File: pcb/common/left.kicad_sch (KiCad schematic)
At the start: 87 parts

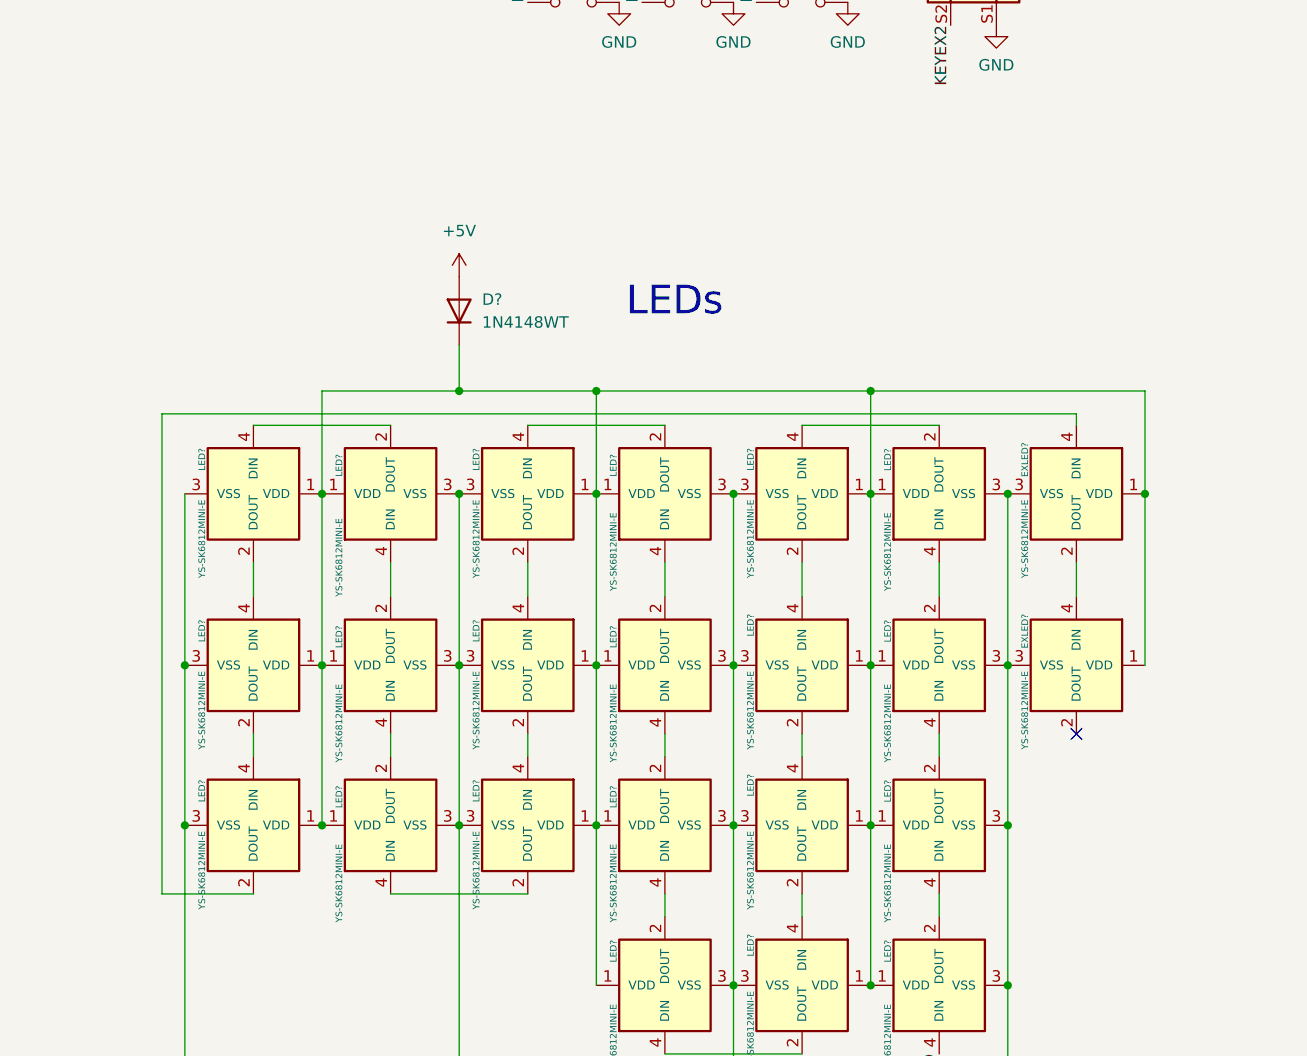
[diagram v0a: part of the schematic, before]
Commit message: Update footprints and sch
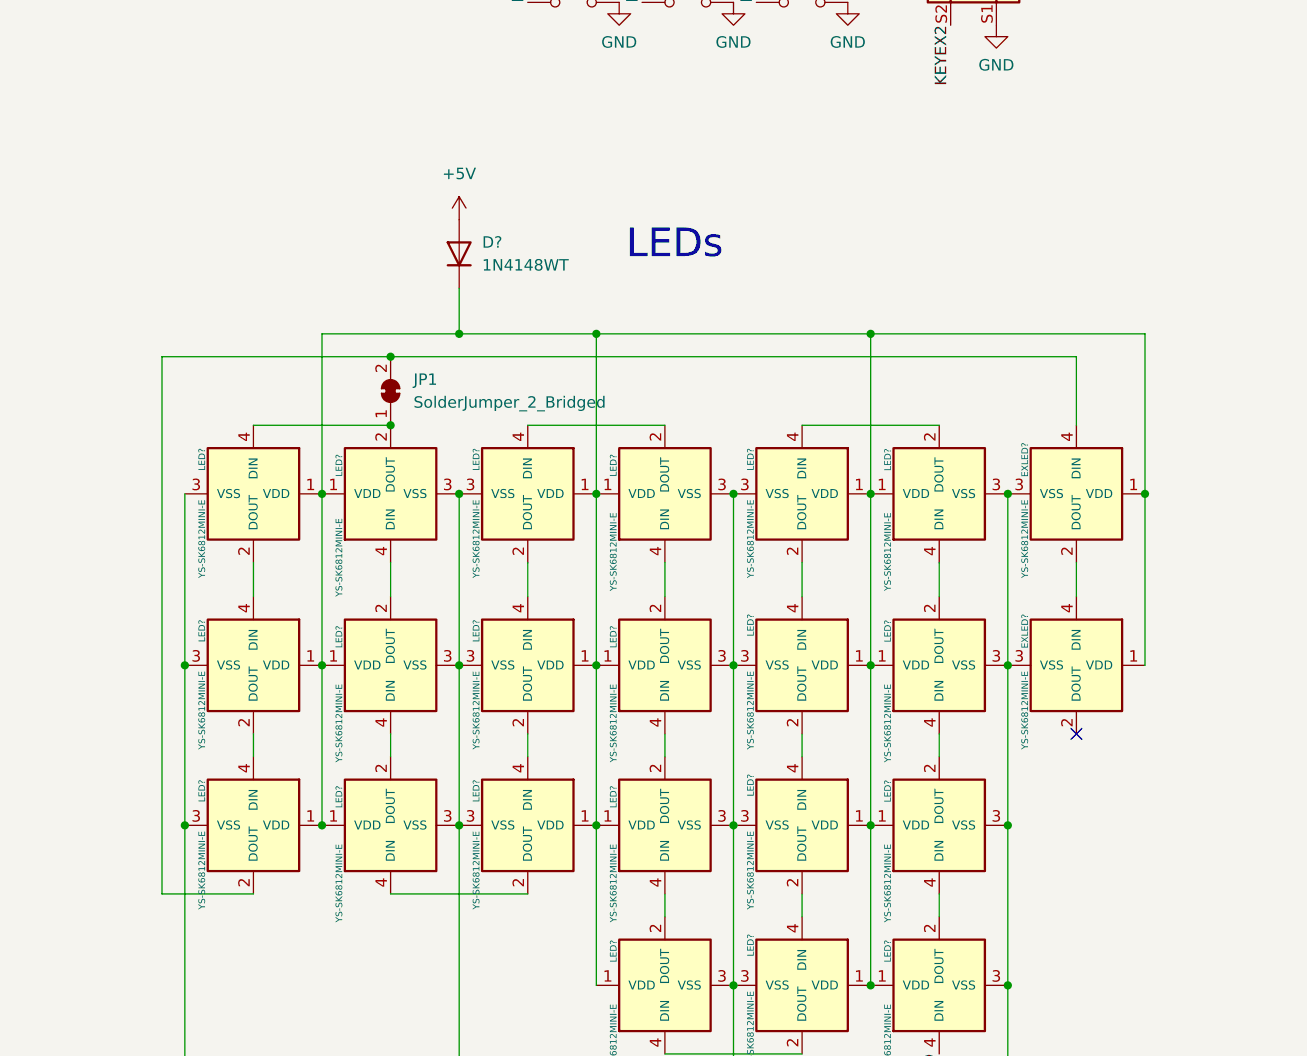
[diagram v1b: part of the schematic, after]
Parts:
- added JP1: SolderJumper_2_Bridged, Jumper:SolderJumper-2_P1.3mm_Open_RoundedPad1.0x1.5mm, symbol Jumper:SolderJumper_2_Bridged
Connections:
- net at LED?.2 (DOUT), LED?.4 (DIN): now also JP1.1 (A)
- net at EXLED?.4 (DIN), LED?.2 (DOUT): now also JP1.2 (B)
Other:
- moved on the sheet: D?
